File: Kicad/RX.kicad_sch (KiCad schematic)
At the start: 29 parts, among them J6 RFShield_OnePiece, Q2 2N7002H, U1 SI4732-A10-GS, Y1 32.768 KHz

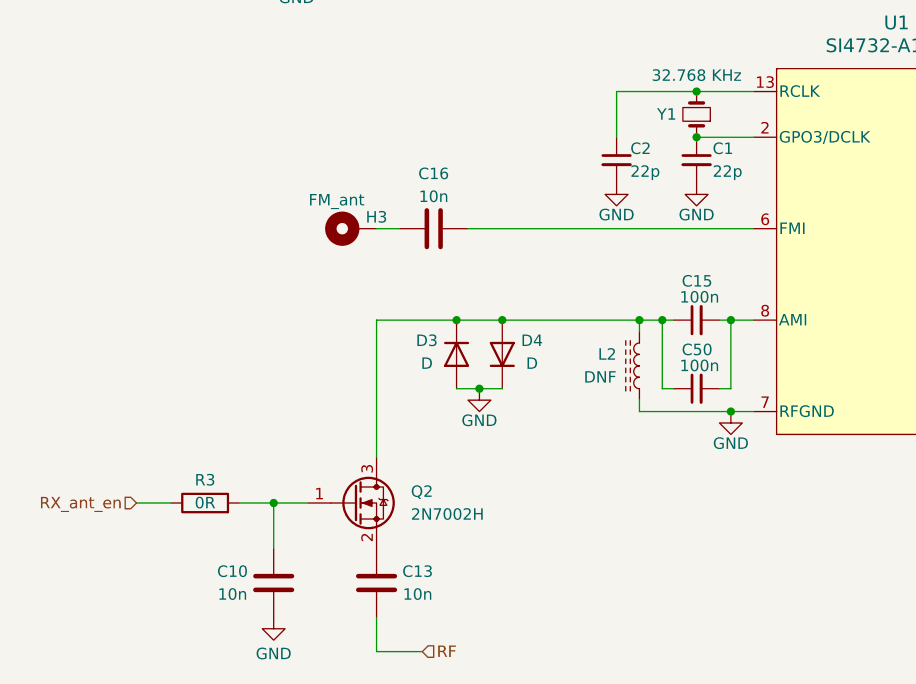
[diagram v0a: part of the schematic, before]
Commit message: Add files via upload
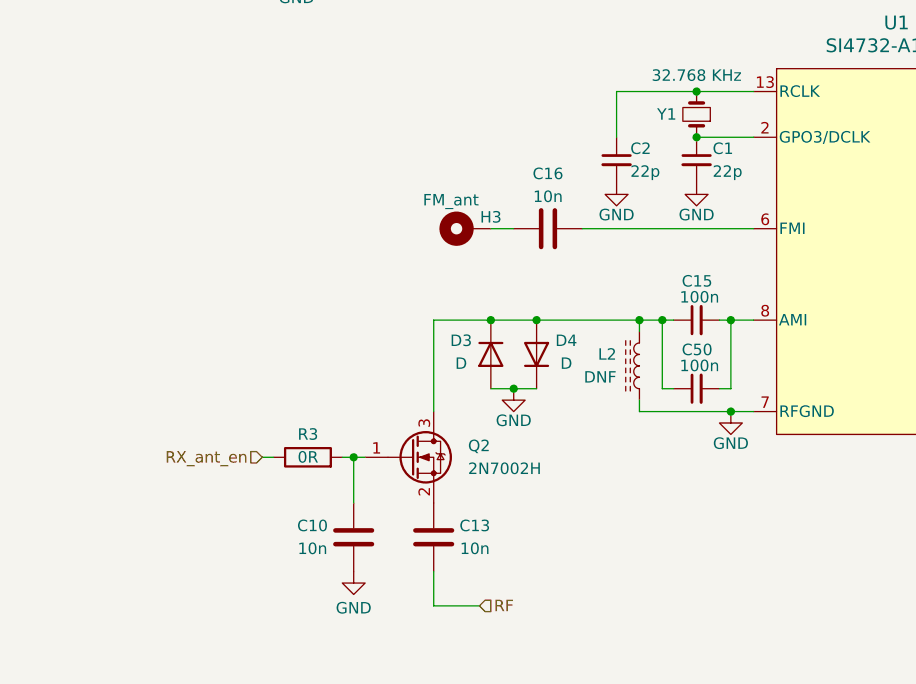
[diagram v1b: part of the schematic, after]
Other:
- moved on the sheet: C10, C13, C16, D3, D4, H3, Q2, R3
